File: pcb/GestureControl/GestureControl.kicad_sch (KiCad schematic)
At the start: 79 parts, among them J1 Conn_01x04_I2I-LCD, J2 BATT, J3 Conn_01x08, J4 Conn_01x06, J5 Conn_01x10, J6 Conn_01x08, SW1 SW1, SW2 SW2, U1 AP5100_3.3, U2 AP5100_3.3

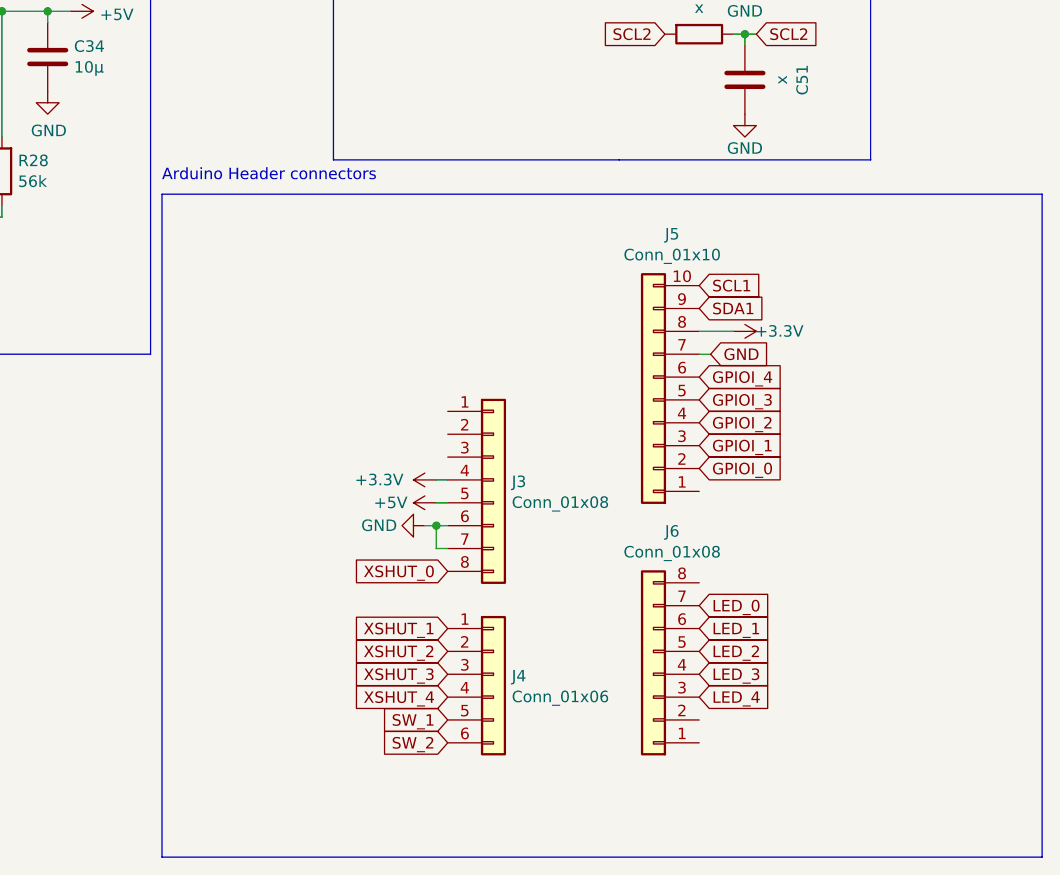
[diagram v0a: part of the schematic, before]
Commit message: add PCBV0.3
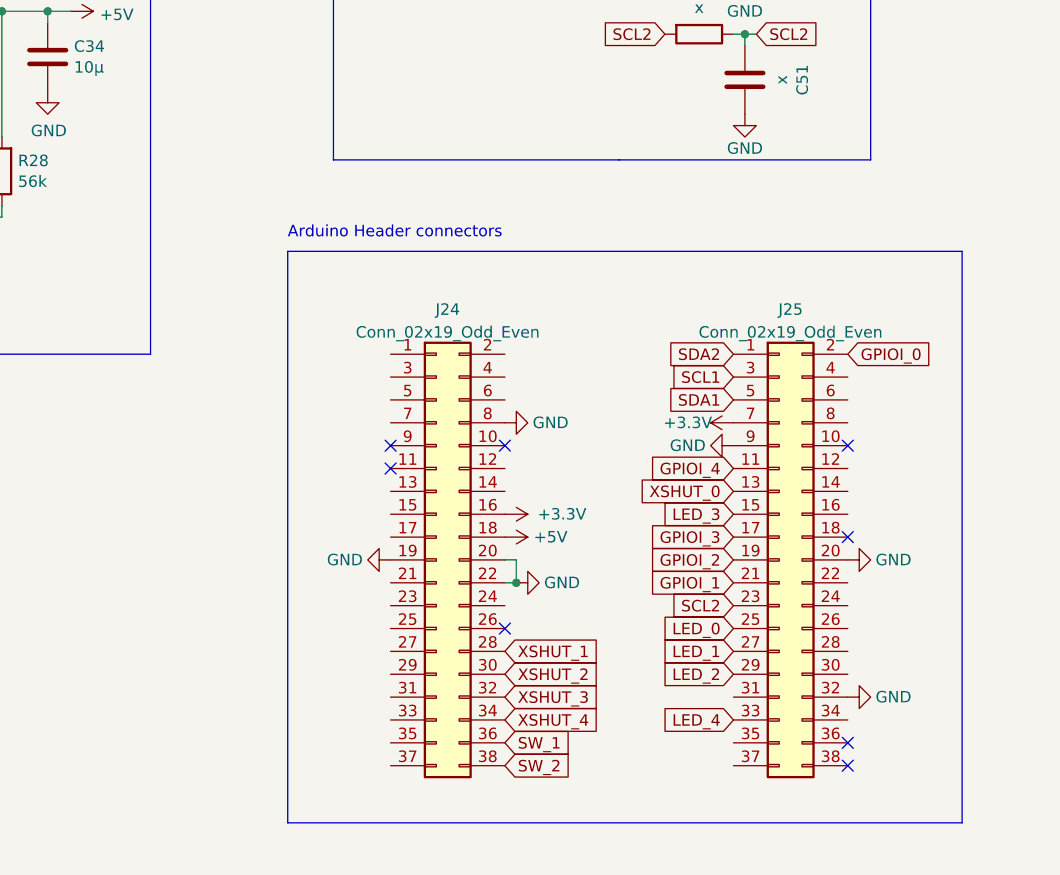
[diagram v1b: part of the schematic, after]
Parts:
- removed J3, J6: Conn_01x08, Connector_PinHeader_2.54mm:PinHeader_1x08_P2.54mm_Vertical, symbol Connector_Generic:Conn_01x08
- removed J4: Conn_01x06, Connector_PinHeader_2.54mm:PinHeader_1x06_P2.54mm_Vertical, symbol Connector_Generic:Conn_01x06
- removed J5: Conn_01x10, Connector_PinHeader_2.54mm:PinHeader_1x10_P2.54mm_Vertical, symbol Connector_Generic:Conn_01x10
- added J24, J25: Conn_02x19_Odd_Even, Connector_PinSocket_2.54mm:PinSocket_2x19_P2.54mm_Vertical, symbol Connector_Generic:Conn_02x19_Odd_Even
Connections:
- net +3V3: now also J24.16 (Pin_16), J25.7 (Pin_7)
- net +5V: now also J24.18 (Pin_18)
- net GND: now also J24.19 (Pin_19), J24.20 (Pin_20), J24.22 (Pin_22), J24.8 (Pin_8), J25.20 (Pin_20), J25.32 (Pin_32), J25.9 (Pin_9)
- net GPIOI_0: now also J25.2 (Pin_2)
- net GPIOI_1: now also J25.21 (Pin_21)
- net GPIOI_2: now also J25.19 (Pin_19)
- net GPIOI_3: now also J25.17 (Pin_17)
- net GPIOI_4: now also J25.11 (Pin_11)
- net LED_0: now also J25.25 (Pin_25)
- net LED_1: now also J25.27 (Pin_27)
- net LED_2: now also J25.29 (Pin_29)
- net LED_3: now also J25.15 (Pin_15)
- net LED_4: now also J25.33 (Pin_33)
- net SCL1: now also J25.3 (Pin_3)
- net SCL2: now also J25.23 (Pin_23)
- net SDA1: now also J25.5 (Pin_5)
- net SDA2: now also J25.1 (Pin_1)
- net SW_1: now also J24.36 (Pin_36)
- net SW_2: now also J24.38 (Pin_38)
- net XSHUT_0: now also J25.13 (Pin_13)
- net XSHUT_1: now also J24.28 (Pin_28)
- net XSHUT_2: now also J24.30 (Pin_30)
- net XSHUT_3: now also J24.32 (Pin_32)
- net XSHUT_4: now also J24.34 (Pin_34)
- no-connect marks 0 -> 8
